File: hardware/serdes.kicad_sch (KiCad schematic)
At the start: 22 parts, among them Q3 BSS138, U4 CCGM1A1, X2 100 MHz LVDS 3.2x2.5

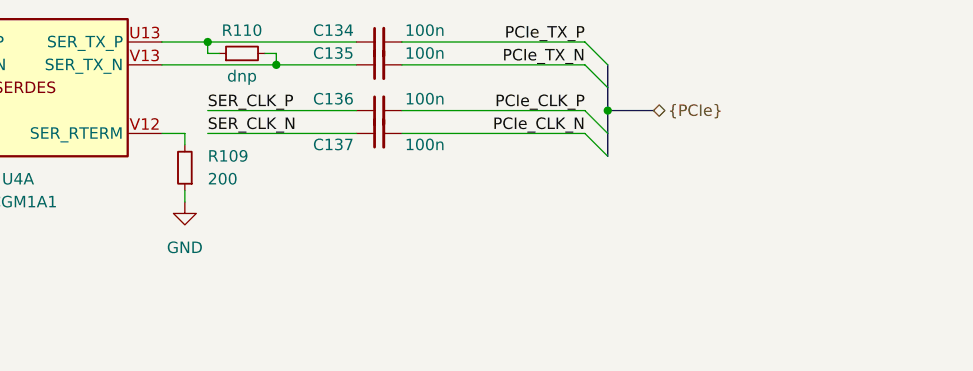
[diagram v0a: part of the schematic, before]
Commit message: routing PCIe
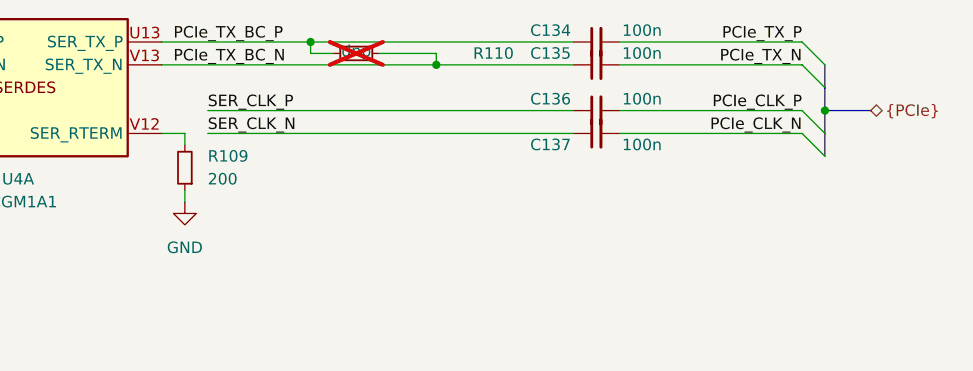
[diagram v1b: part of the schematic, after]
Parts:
- R110: now not fitted
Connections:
- net PCIe_TX_BC_P: now reaches C134.1, R110.1, U4.U13 (SER_TX_P)
- net PCIe_TX_BC_N: now reaches C135.1, R110.2, U4.V13 (SER_TX_N)
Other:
- moved on the sheet: C134, C135, C136, C137
